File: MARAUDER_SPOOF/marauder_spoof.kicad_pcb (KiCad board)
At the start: 2 copper layers, 67 x 23.3 mm, 25 parts, among them J1 Coil, J2 Conn_01x10_Socket, J3 Conn_01x08_Socket, J4 Conn_01x08_Socket, J5 Conn_01x10_Socket, U1 TC4424

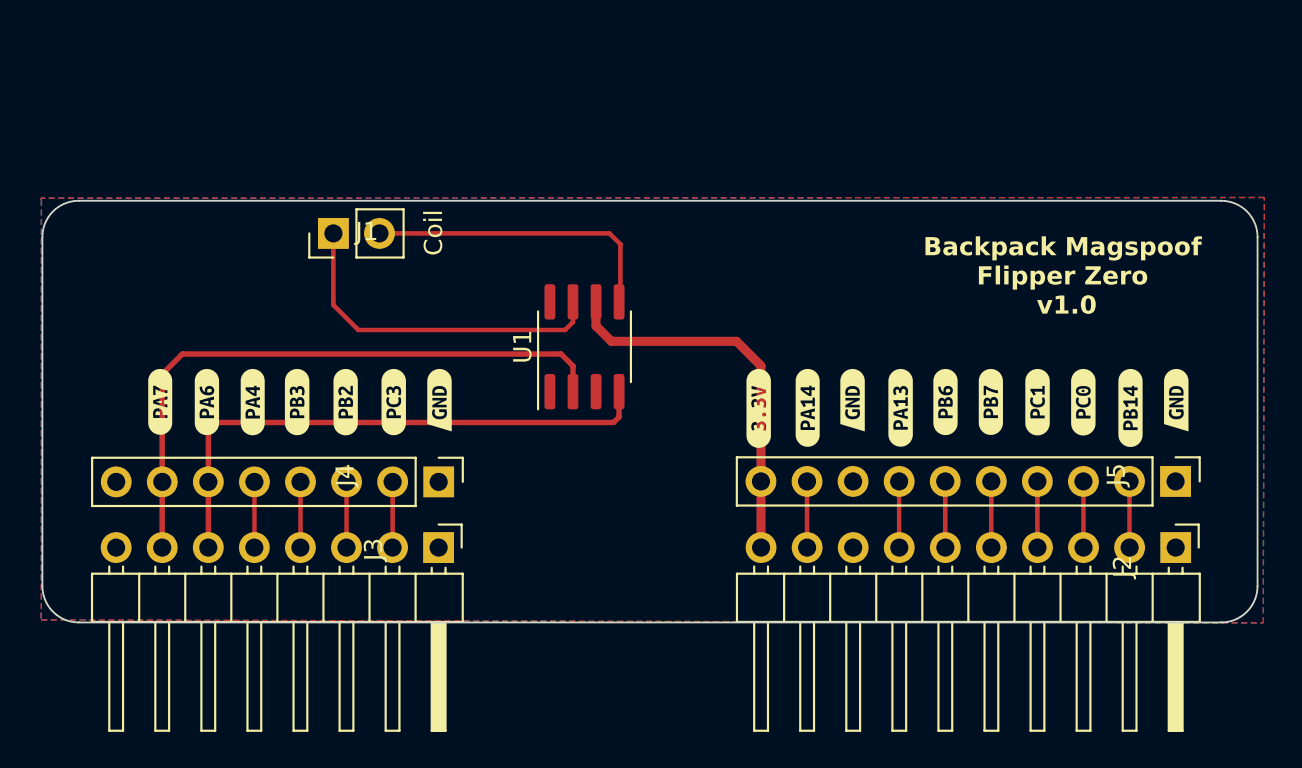
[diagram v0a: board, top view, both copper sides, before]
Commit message: update layout magspoof-wifi
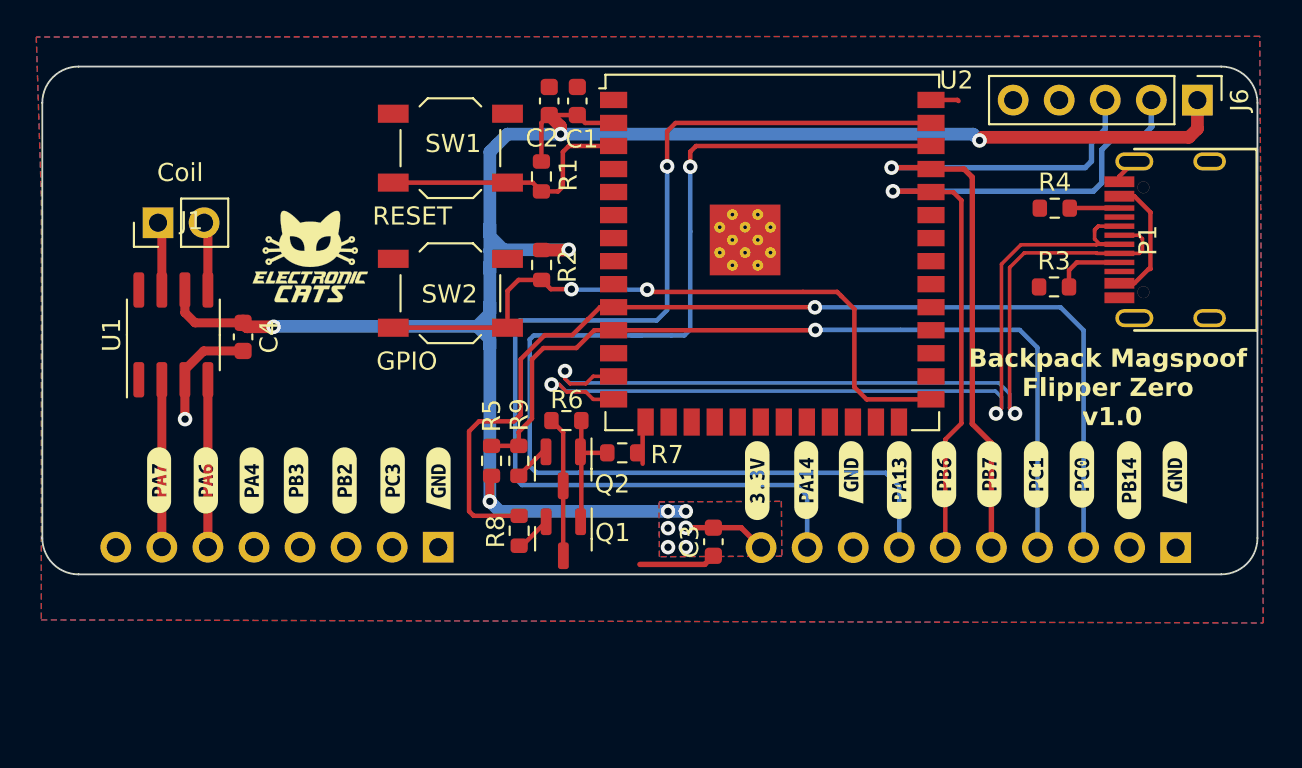
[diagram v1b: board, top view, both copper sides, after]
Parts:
- removed J4: Conn_01x08_Socket, Connector_PinHeader_2.54mm:PinHeader_1x08_P2.54mm_Vertical
- removed J5: Conn_01x10_Socket, Connector_PinHeader_2.54mm:PinHeader_1x10_P2.54mm_Vertical
- added C1: 1uF, Capacitor_SMD:C_0603_1608Metric, F.Cu at (225.5, 57.9)
- added C2: 10uF, Capacitor_SMD:C_0603_1608Metric, F.Cu at (223.9, 57.9)
- added C3: 10uF, Capacitor_SMD:C_0603_1608Metric, F.Cu at (233.0, 82.2)
- added C4: 10uF, Capacitor_SMD:C_0603_1608Metric, F.Cu at (207.1, 70.9)
- added G***: LOGO, Aesthetics:electronic_cats_logo_4x3, F.Cu at (210.8, 66.5)
- added J6: GPS, Connector_PinHeader_2.54mm:PinHeader_1x05_P2.54mm_Vertical, F.Cu at (259.7, 57.9)
- added P1: USB_C_Plug_USB2.0, Connectors:C393939, F.Cu at (256.2, 65.5)
- added Q1: DMP2004TK-7, Package_TO_SOT_SMD:SOT-23, F.Cu at (224.7, 82.0)
- added Q2: DMP2004TK-7, Package_TO_SOT_SMD:SOT-23, F.Cu at (224.7, 78.2)
- added R1: 10K, Resistor_SMD:R_0603_1608Metric, F.Cu at (223.5, 62.1)
- added R2: 10K, Resistor_SMD:R_0603_1608Metric, F.Cu at (223.5, 66.9)
- added R3: 5k1, Resistor_SMD:R_0603_1608Metric, F.Cu at (251.8, 68.2)
- added R4: 5k1, Resistor_SMD:R_0603_1608Metric, F.Cu at (251.8, 63.8)
- added R5: 10K, Resistor_SMD:R_0603_1608Metric, F.Cu at (220.8, 77.7)
- added R6: 10K, Resistor_SMD:R_0603_1608Metric, F.Cu at (224.9, 75.5)
- added R7: 150, Resistor_SMD:R_0603_1608Metric, F.Cu at (228.0, 77.3)
- added R8: 4k7, Resistor_SMD:R_0603_1608Metric, F.Cu at (222.3, 81.6)
- added R9: 4k7, Resistor_SMD:R_0603_1608Metric, F.Cu at (222.3, 77.7)
- added SW1: RESET, Button_Switch_SMD:SW_SPST_TL3342, F.Cu at (218.5, 60.5)
- added SW2: GPIO, Button_Switch_SMD:SW_SPST_TL3342, F.Cu at (218.5, 68.5)
- added U2: ESP32-S3-WROOM-1U-N16, RF_Module:ESP32-S3-WROOM-1U, F.Cu at (236.2, 66.2)
- J2: footprint Connector_PinHeader_2.54mm:PinHeader_1x10_P2.54mm_Horizontal -> Connector_PinHeader_2.54mm:PinHeader_1x10_P2.54mm_Vertical; moved to B.Cu
- J3: footprint Connector_PinHeader_2.54mm:PinHeader_1x08_P2.54mm_Horizontal -> Connector_PinHeader_2.54mm:PinHeader_1x08_P2.54mm_Vertical; moved to B.Cu
- moved U1 22.7 mm to (203.2, 70.8)
- moved G*** 12.9 mm to (241.2, 65.2)
- moved J1 9.69 mm to (202.4, 64.6)
- moved REF** 9.01 mm to (211.7, 66.5)
- moved kibuzzard-6488EEAF 4.32 mm to (217.8, 78.7)
- moved kibuzzard-648B91CB 4.32 mm to (207.5, 78.8)
- moved kibuzzard-648B91E6 4.32 mm to (210.0, 78.8)
- moved kibuzzard-648B921B 4.32 mm to (215.3, 78.8)
- moved kibuzzard-648B922F 4.32 mm to (202.4, 78.8)
- moved kibuzzard-648B923F 4.32 mm to (205.0, 78.8)
- moved kibuzzard-648B91FC 4.32 mm to (212.7, 78.8)
- moved kibuzzard-6488EEAF 3.98 mm to (240.6, 78.4)
- moved kibuzzard-648B93E0 3.98 mm to (245.7, 78.5)
- moved kibuzzard-648B93EF 3.98 mm to (250.8, 78.5)
- moved kibuzzard-6488EEAF 3.98 mm to (258.4, 78.4)
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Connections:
- J2 pad 3: /PC0 -> /LPUART_RX
- J2 pad 4: /PC1 -> /LPUART_TX
- J2 pad 5: /PB7 -> /RX
- J2 pad 6: /PB6 -> /TX
- J2 pad 7: /PA13 -> /SWDIO
- J2 pad 9: /PA14 -> /SWCLK
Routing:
- net +3V3: track 21.4 -> 116.4 mm, vias 0 -> 11
- net /SWDIO: track 0.00 -> 64.0 mm, vias 0 -> 1
- net /SWCLK: track 0.00 -> 61.1 mm, vias 0 -> 1
- net /LPUART_RX: track 0.00 -> 58.3 mm, vias 0 -> 1
- net /D+: track 0.00 -> 48.9 mm, vias 0 -> 2
- net /D-: track 0.00 -> 47.8 mm, vias 0 -> 2
- net /LPUART_TX: track 0.00 -> 46.6 mm, vias 0 -> 1
- net /TX: track 0.00 -> 41.8 mm, vias 0 -> 1
- net /RX: track 0.00 -> 40.4 mm, vias 0 -> 1
- net /BOOT: track 0.00 -> 37.2 mm, vias 0 -> 2
- net /IN_A: track 34.4 -> 9.23 mm
- net /IN_B: track 30.8 -> 9.24 mm
- net /Out_A: track 19.0 -> 3.80 mm
- net /RST: track 0.00 -> 14.5 mm
- net GND: track 0.00 -> 13.6 mm, vias 0 -> 1
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- added copper zone on B.Cu, net +3V3
- added copper zone on F.Cu, net +3V3
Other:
- board size 67 x 23.3 mm -> 67 x 28 mm
